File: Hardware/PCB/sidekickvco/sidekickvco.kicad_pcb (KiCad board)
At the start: 2 copper layers, 169.5 x 163 mm, 123 parts, among them J1 Conn_02x04_Odd_Even, J14 Wire pad, J15 Wire pad, J16 Wire pad, J17 Wire pad, J18 AudioJack2, J19 AudioJack2, J2 3_pin_Molex_header, J20 Synth_power_2x5, J21 AudioJack2, J22 AudioJack2, J3 3_pin_Molex_header, J4 4_pin_Molex_header, J5 2_pin_Molex_header, J6 2_pin_Molex_header, J7 2_pin_Molex_header, Q1 2N3904, Q2 2N3904, SW2 SW_DP3T, U1 TL072, U2 AS3340A, U3 LM4040BIZ-5, U4 LM4040BIZ-5, U5 L79L05_TO92, U6 TL074

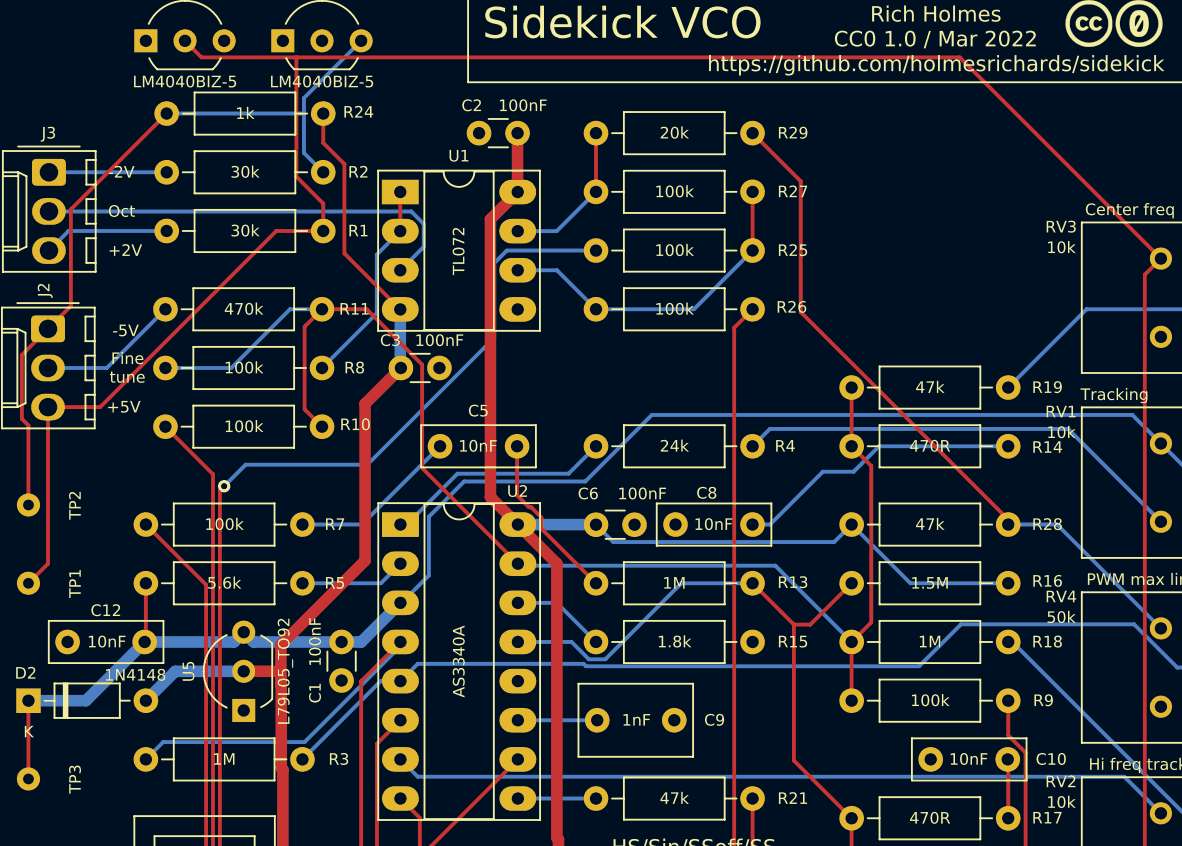
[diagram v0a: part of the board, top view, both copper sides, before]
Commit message: Matching notes on silk
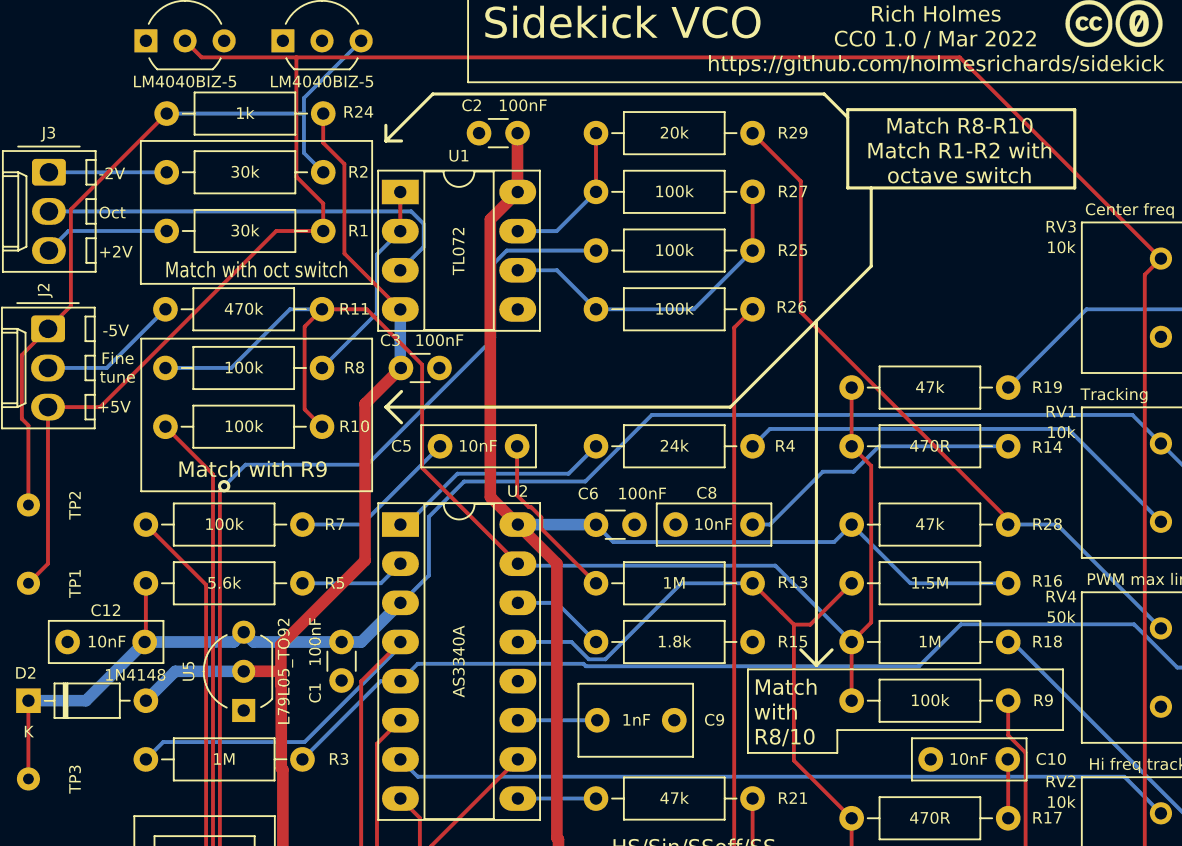
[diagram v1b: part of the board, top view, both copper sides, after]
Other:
- board text added: "Match R8-R10 Match R1-R2 with octave switch"
- board text added: "Match with R8/10"
- board text added: "Match with R9"
- board text added: "Match with oct switch"
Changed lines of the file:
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@@
     (property "Vendor" "Tayda")
     (attr through_hole)
-    (fp_text reference "R10" (at -2.159 0.127) (layer "F.SilkS")
+    (fp_text reference "R10" (at -2.112 0) (layer "F.SilkS")
       (effects (font (size 0.75 0.75) (thickness 0.15)))
     )
@@
     (property "Vendor" "Tayda")
     (attr through_hole)
-    (fp_text reference "C5" (at 2.5 2.286) (layer "F.SilkS")
+    (fp_text reference "C5" (at 7.5 0) (layer "F.SilkS")
       (effects (font (size 0.75 0.75) (thickness 0.15)))
     )
@@
       (net 2 "-5V") (pinfunction "1") (pintype "passive"))
   )
+  (gr_line (start 124.052 44.24) (end 149.452 44.24) (layer "F.SilkS") (width 0.2))
+  (gr_rect (start 105.129 60.115) (end 120.115 70.021) (layer "F.SilkS") (width 0.12) (fill none))
+  (gr_line (start 152.5 55.416) (end 152.5 50.336) (layer "F.SilkS") (width 0.2))
+  (gr_line (start 150.3 87) (end 150.3 85.5205) (layer "F.SilkS") (width 0.12))
   (gr_rect (start 126.338 37.382) (end 173.963 43.478) (layer "F.SilkS") (width 0.12) (fill none))
+  (gr_rect (start 105.1036 47.288) (end 120.115 56.559) (layer "F.SilkS") (width 0.12) (fill none))
+  (gr_line (start 121.004 46.272) (end 121.004 47.288) (layer "F.SilkS") (width 0.2))
+  (gr_line (start 149.452 44.24) (end 150.976 45.764) (layer "F.SilkS") (width 0.2))
+  (gr_line (start 121.004 64.56) (end 143.356 64.56) (layer "F.SilkS") (width 0.2))
+  (gr_line (start 148.944 81.324) (end 148.944 58.972) (layer "F.SilkS") (width 0.2))
+  (gr_line (start 147.928 80.308) (end 148.944 81.324) (layer "F.SilkS") (width 0.2))
+  (gr_line (start 121.004 64.56) (end 122.02 65.576) (layer "F.SilkS") (width 0.2))
+  (gr_line (start 122.02 63.544) (end 121.004 64.56) (layer "F.SilkS") (width 0.2))
+  (gr_line (start 144.499 81.578) (end 144.499 87) (layer "F.SilkS") (width 0.12))
+  (gr_line (start 150.3 85.515) (end 164.946 85.515) (layer "F.SilkS") (width 0.12))
+  (gr_line (start 164.946 85.515) (end 164.946 81.578) (layer "F.SilkS") (width 0.12))
+  (gr_line (start 121.004 47.288) (end 122.02 47.288) (layer "F.SilkS") (width 0.2))
+  (gr_line (start 143.356 64.56) (end 152.5 55.416) (layer "F.SilkS") (width 0.2))
+  (gr_line (start 124.052 44.24) (end 121.004 47.288) (layer "F.SilkS") (width 0.2))
+  (gr_rect (start 150.976 45.256) (end 165.708 50.336) (layer "F.SilkS") (width 0.2) (fill none))
+  (gr_line (start 164.946 81.578) (end 144.499 81.578) (layer "F.SilkS") (width 0.12))
+  (gr_line (start 144.499 87) (end 150.3 87) (layer "F.SilkS") (width 0.12))
+  (gr_line (start 149.96 80.308) (end 148.944 81.324) (layer "F.SilkS") (width 0.2))
   (gr_line (start 76.3 25) (end 76.3 33) (layer "Dwgs.User") (width 0.1))
   (gr_line (start 72.3 29) (end 80.3 29) (layer "Dwgs.User") (width 0.1))
@@
     (effects (font (size 1 1) (thickness 0.15)))
   )
-  (gr_text "+2V" (at 102.97 54.4) (layer "F.SilkS")
+  (gr_text "Match with oct switch\n" (at 112.622 55.67) (layer "F.SilkS")
+    (effects (font (size 1 0.8) (thickness 0.15)))
+  )
+  (gr_text "+2V" (at 102.3604 54.5016) (layer "F.SilkS")
     (effects (font (size 0.75 0.75) (thickness 0.15)) (justify left))
   )
-  (gr_text "-5V" (at 104.113 59.607) (layer "F.SilkS")
+  (gr_text "-5V" (at 103.478 59.607) (layer "F.SilkS")
     (effects (font (size 0.75 0.75) (thickness 0.15)))
   )
@@
     (effects (font (size 1 1) (thickness 0.15)))
   )
+  (gr_text "Match\nwith\nR8/10" (at 144.88 84.372) (layer "F.SilkS")
+    (effects (font (size 1 1) (thickness 0.15)) (justify left))
+  )
+  (gr_text "Match R8-R10\nMatch R1-R2 with\noctave switch" (at 158.2404 47.9484) (layer "F.SilkS")
+    (effects (font (size 1 1) (thickness 0.15)))
+  )
   (gr_text "SS" (at 29.31 110.915 90) (layer "F.SilkS")
     (effects (font (size 1 1) (thickness 0.15)) (justify right))
   )
-  (gr_text "Fine\ntune" (at 104.24 62.02) (layer "F.SilkS")
+  (gr_text "Fine\ntune" (at 103.605 62.02) (layer "F.SilkS")
     (effects (font (size 0.75 0.75) (thickness 0.15)))
   )
+  (gr_text "Match with R9" (at 112.368 68.624) (layer "F.SilkS")
+    (effects (font (size 1 1) (thickness 0.15)))
+  )
   (gr_text "HS" (at 17.88 110.915 90) (layer "F.SilkS")
     (effects (font (size 1 1) (thickness 0.15)) (justify right))
@@
     (effects (font (size 1 1) (thickness 0.15)))
   )
-  (gr_text "-2V" (at 102.97 49.32) (layer "F.SilkS")
+  (gr_text "-2V" (at 102.3604 49.4216) (layer "F.SilkS")
     (effects (font (size 0.75 0.75) (thickness 0.15)) (justify left))
   )
-  (gr_text "Oct" (at 102.97 51.86) (layer "F.SilkS")
+  (gr_text "Oct" (at 102.3604 51.9616) (layer "F.SilkS")
     (effects (font (size 0.75 0.75) (thickness 0.15)) (justify left))
   )
@@
     (effects (font (size 1 1) (thickness 0.15)))
   )
-  (gr_text "+5V" (at 103.986 64.56) (layer "F.SilkS")
+  (gr_text "+5V" (at 103.351 64.56) (layer "F.SilkS")
     (effects (font (size 0.75 0.75) (thickness 0.15)))
   )
